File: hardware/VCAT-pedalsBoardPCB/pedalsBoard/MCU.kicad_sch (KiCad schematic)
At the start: 0 parts

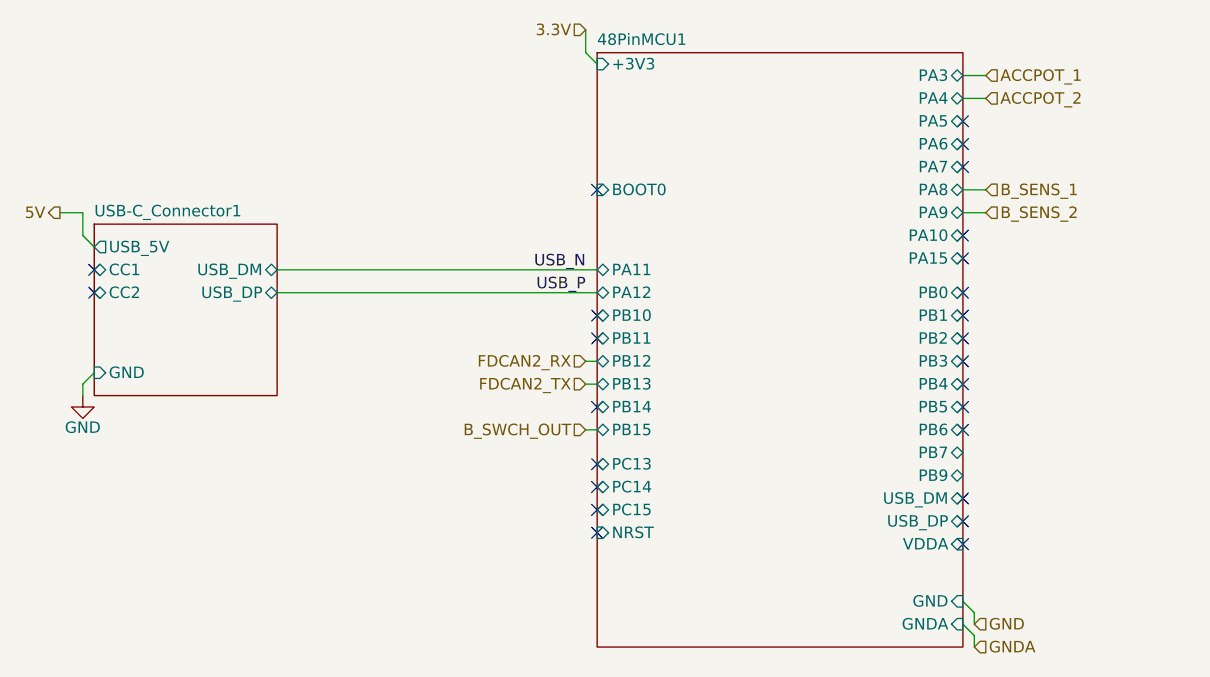
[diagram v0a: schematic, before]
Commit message: test
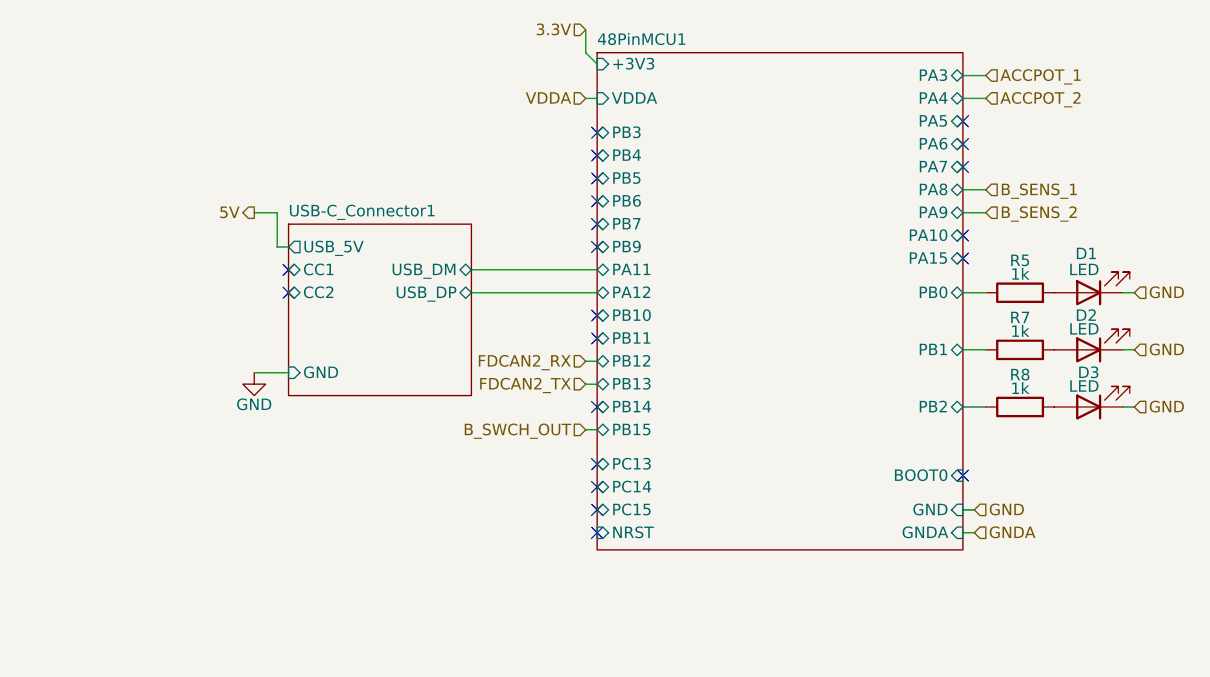
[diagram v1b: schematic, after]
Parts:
- added D1: LED, LHRS_Special:RGB_LED, symbol Device:LED
- added D2, D3: LED, symbol Device:LED
- added R5, R7, R8: 1k, Resistor_SMD:R_0603_1608Metric, symbol Device:R
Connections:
- net 48PinMCU1/PB0: now also R5.1
- net 48PinMCU1/PB1: now also R7.1
- net 48PinMCU1/PB2: now also R8.1
- net GND: now also D1.1 (K), D2.1 (K), D3.1 (K)
- new net: D3.2 (A), R8.2
- new net: D1.2 (A), R5.2
- new net: D2.2 (A), R7.2
- no-connect marks 25 -> 21
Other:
- sheet 48PinMCU1 ports: added none; removed USB_DM, USB_DP
